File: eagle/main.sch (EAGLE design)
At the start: 34 parts, among them Q1 BSS97, Q2 BSS97, Q3 BSS97, Q4 BSS97, U1 LTC3789EGNPBF

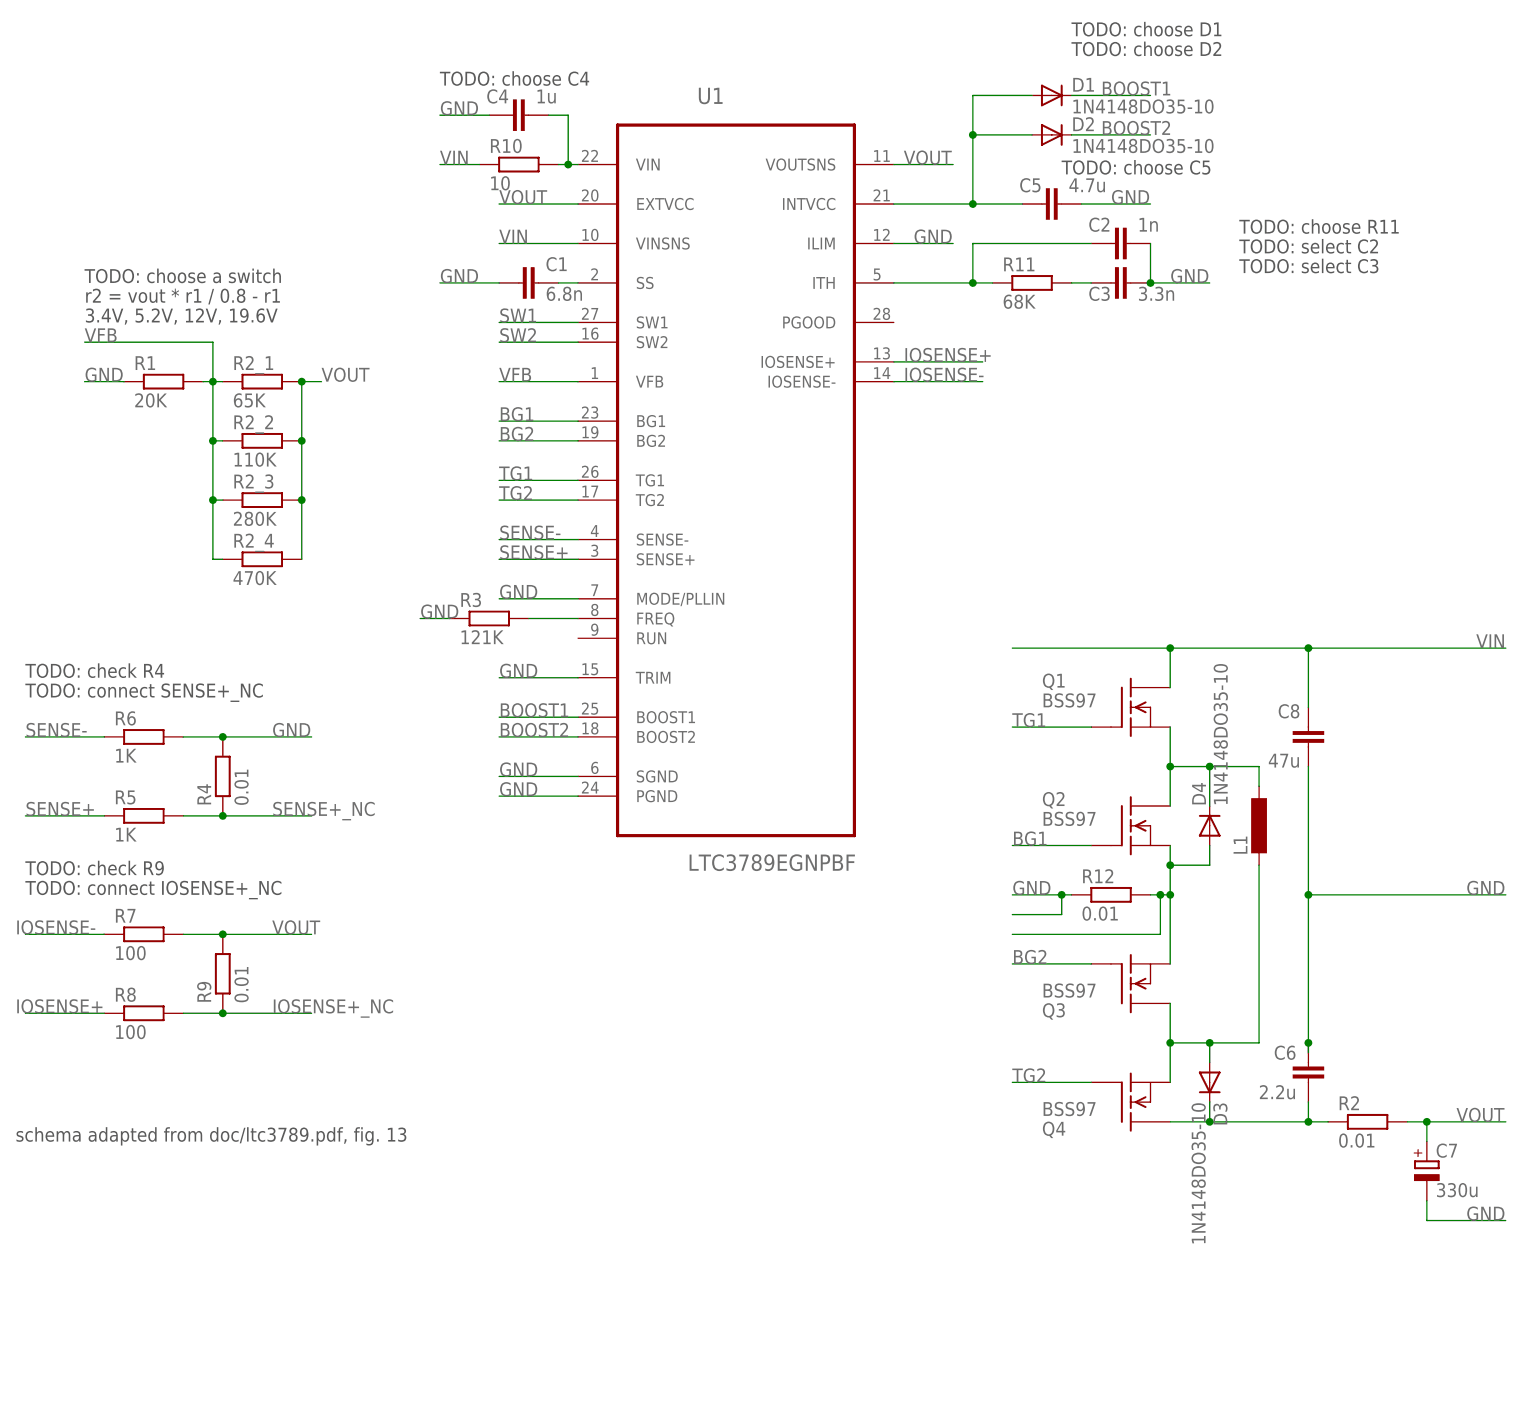
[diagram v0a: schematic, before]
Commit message: [ update ] sch
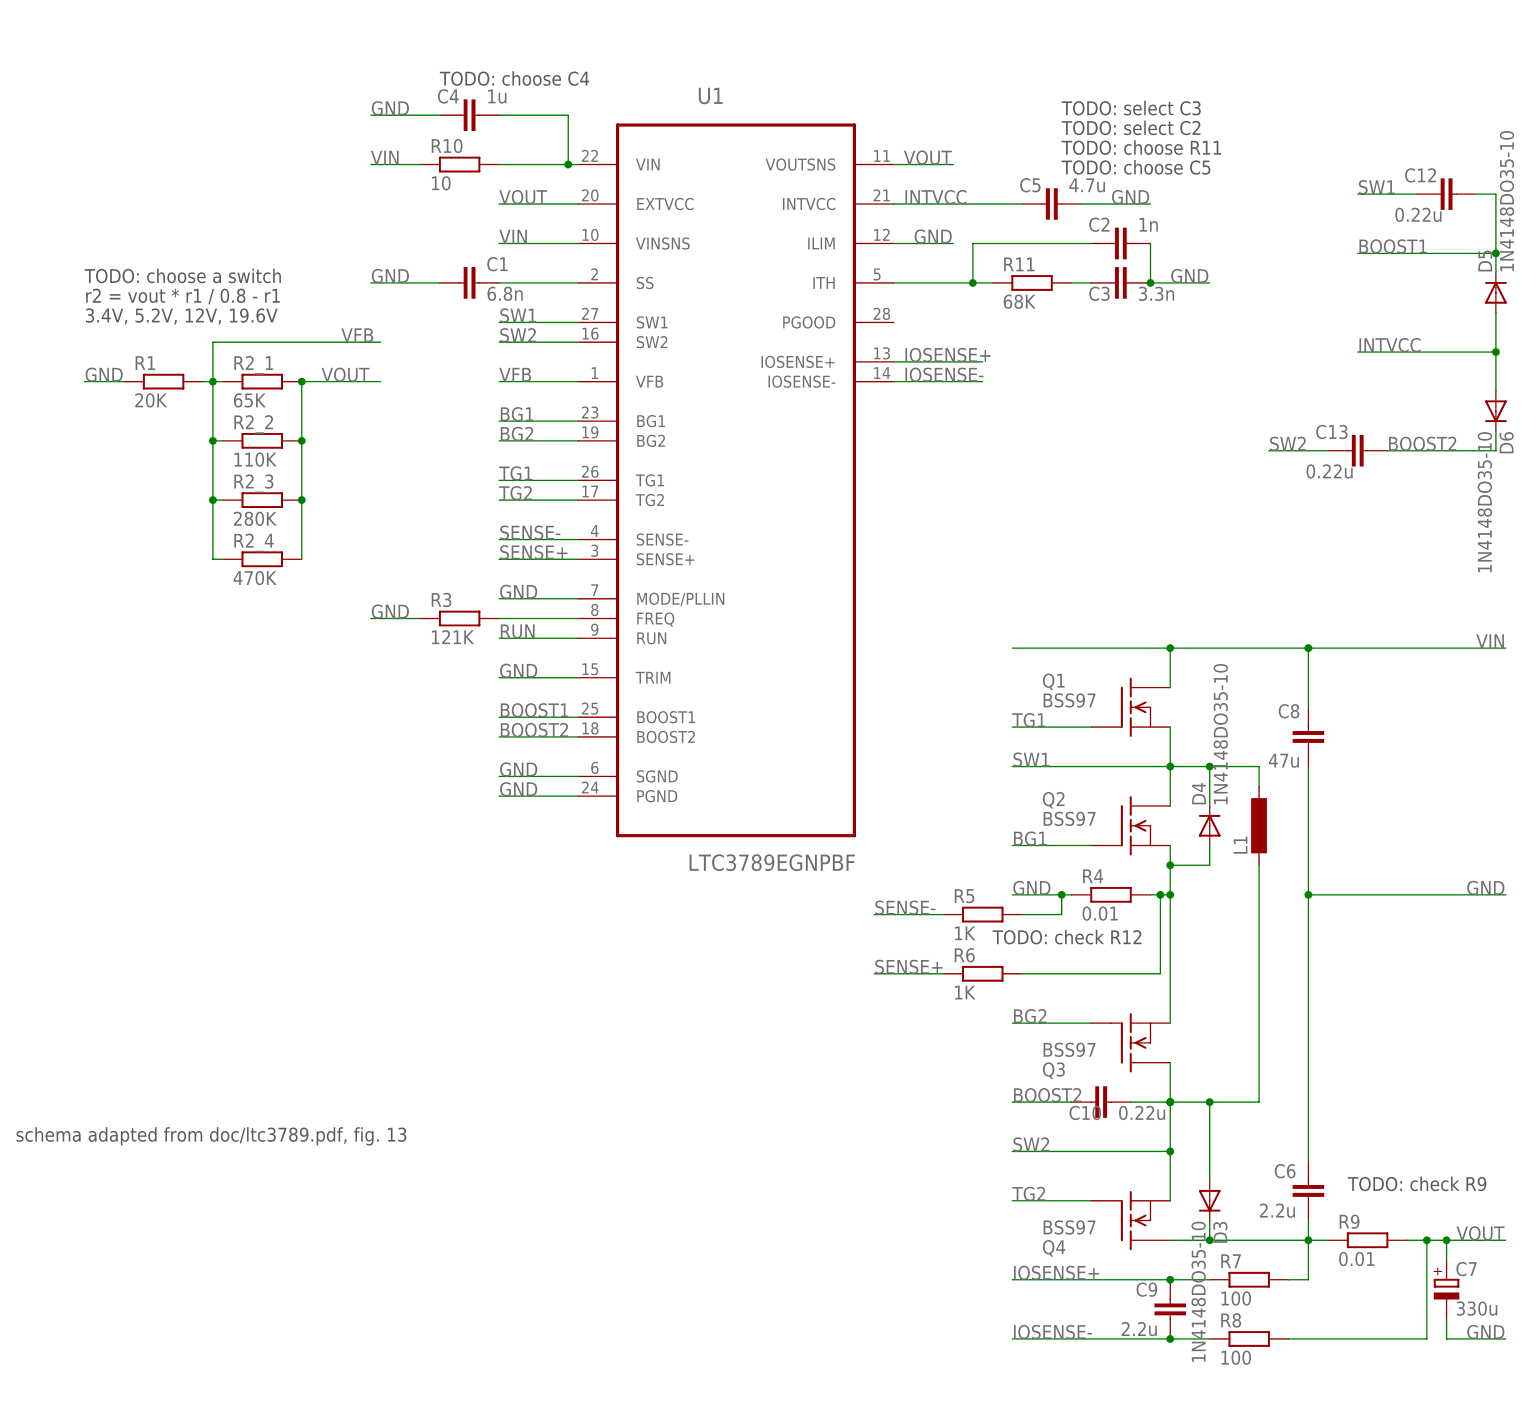
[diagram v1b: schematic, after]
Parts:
- removed D1, D2: 1N4148DO35-10, diode:1N4148DO35-10
- removed R12, R2: 0.01, resistor:R-EU_R1206
- added C10, C12, C13: 0.22u, rcl:C-EUC1206K
- added C9: 2.2u, rcl:C-EUC1206K
- added D5, D6: 1N4148DO35-10, diode:1N4148DO35-10
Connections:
- removed net IOSENSE+_NC: R8.2, R9.1
- removed net N$11: D4.C, L1.1, Q1.S, Q2.D
- removed net N$6: C5.1, D1.A, D2.A, U1.INTVCC
- removed net N$8: D3.A, L1.2, Q3.D, Q4.S
- removed net SENSE+_NC: R4.1, R5.2
- new net INTVCC: C5.1, D5.A, D6.A, U1.INTVCC
- new net RUN: U1.RUN
- net BOOST1: now also C12.2, D5.C; no longer D1.C
- net BOOST2: now also C10.1, C13.2, D6.C; no longer D2.C
- net GND: now also R4.1, R5.2; no longer R12.1, R4.2, R6.2
- net IOSENSE+: now also C9.2, R7.1; no longer R8.1
- net IOSENSE-: now also C9.1, R8.1; no longer R7.1
- net N$7: now also R7.2, R9.1; no longer R2.1
- net N$9: now also R4.2, R6.2; no longer R12.2
- net SENSE+: now also R6.1; no longer R5.1
- net SENSE-: now also R5.1; no longer R6.1
- net SW1: now also C12.1, D4.C, L1.1, Q1.S, Q2.D
- net SW2: now also C10.2, C13.1, D3.A, L1.2, Q3.D, Q4.S
- net VOUT: now also R8.2; no longer R2.2, R7.2
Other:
- note added: "TODO: check R12"
- note removed: "TODO: check R4"
- note removed: "TODO: choose D1"
- note removed: "TODO: choose D2"
- note removed: "TODO: connect IOSENSE+_NC"
- note removed: "TODO: connect SENSE+_NC"
- moved on the sheet: C1, C4, C6, C7, D3, Q3, Q4, R10, R3, R4, R5, R6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
